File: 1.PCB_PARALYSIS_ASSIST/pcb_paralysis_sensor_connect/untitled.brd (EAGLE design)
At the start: 160 x 100 mm, 7 parts

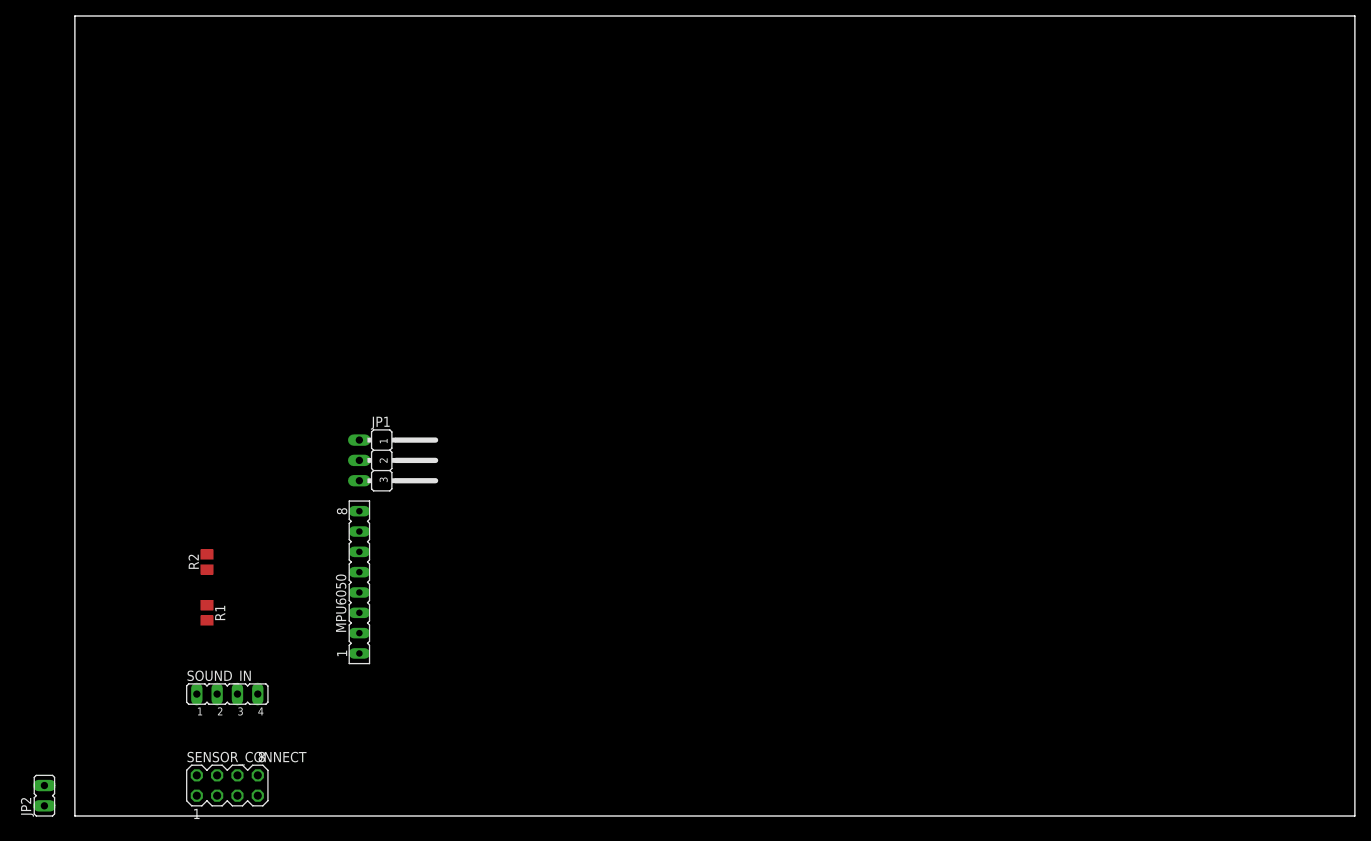
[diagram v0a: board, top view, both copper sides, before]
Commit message: small board
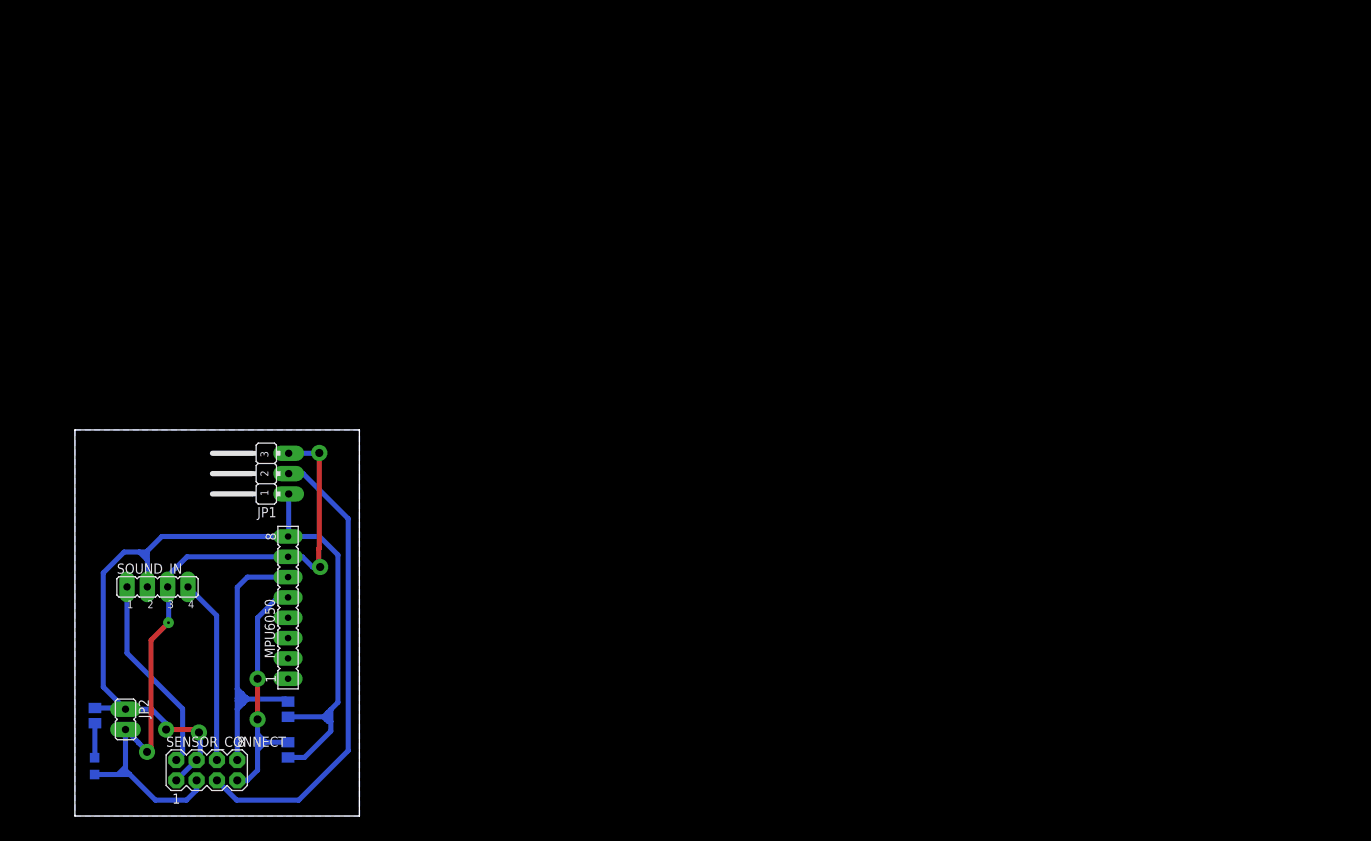
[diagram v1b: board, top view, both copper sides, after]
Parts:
- added LED1: (no value), led:CHIP-LED0805
- added R3: 1k, adafruit:M0805
- moved R2 21.0 mm to (26.6, 13.3), flipped to the bottom
- moved R1 19.9 mm to (26.6, 8.27), flipped to the bottom, turned to 90 degrees
- moved SOUND_IN 16.0 mm to (10.3, 28.6)
- moved JP2 13.9 mm to (6.32, 12.1), turned to 180 degrees
- moved JP1 11.5 mm to (25.5, 42.8), turned to 90 degrees
- moved MPU6050 9.46 mm to (26.6, 26.0)
- moved SENSOR_CONNECT 3.20 mm to (16.5, 5.73)
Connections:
- removed net N$2: SENSOR_CONNECT.5
- removed net N$3: SENSOR_CONNECT.3
- removed net N$4: SENSOR_CONNECT.1
- removed net N$5: SENSOR_CONNECT.8
- removed net N$6: SENSOR_CONNECT.6
- removed net N$7: SENSOR_CONNECT.4
- removed net N$8: SENSOR_CONNECT.2
- net 5V: now also R3.1, SENSOR_CONNECT.1, SENSOR_CONNECT.4
- net GND: now also LED1.C, SENSOR_CONNECT.3
- net N$1: now also LED1.A, R3.2; no longer SENSOR_CONNECT.7
- net SCL: now also SENSOR_CONNECT.8
- net SDA: now also SENSOR_CONNECT.7
- net SOUND_A0: now also SENSOR_CONNECT.6
- net SOUND_D0: now also SENSOR_CONNECT.2
- net TEMP_DATA: now also SENSOR_CONNECT.5
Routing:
- net 5V: track 0.00 -> 120.4 mm, vias 0 -> 2
- net GND: track 0.00 -> 90.7 mm, vias 0 -> 4
- net TEMP_DATA: track 0.00 -> 58.8 mm
- net SCL: track 0.00 -> 41.8 mm
- net SDA: track 0.00 -> 33.5 mm, vias 0 -> 2
- net SOUND_D0: track 0.00 -> 24.8 mm
- net SOUND_A0: track 0.00 -> 23.1 mm
- net N$1: track 0.00 -> 4.33 mm
- added copper zone on layer 16, net GND
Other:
- board size 160 x 100 mm -> 35.6 x 48.3 mm
